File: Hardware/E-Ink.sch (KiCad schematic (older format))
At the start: 0 parts

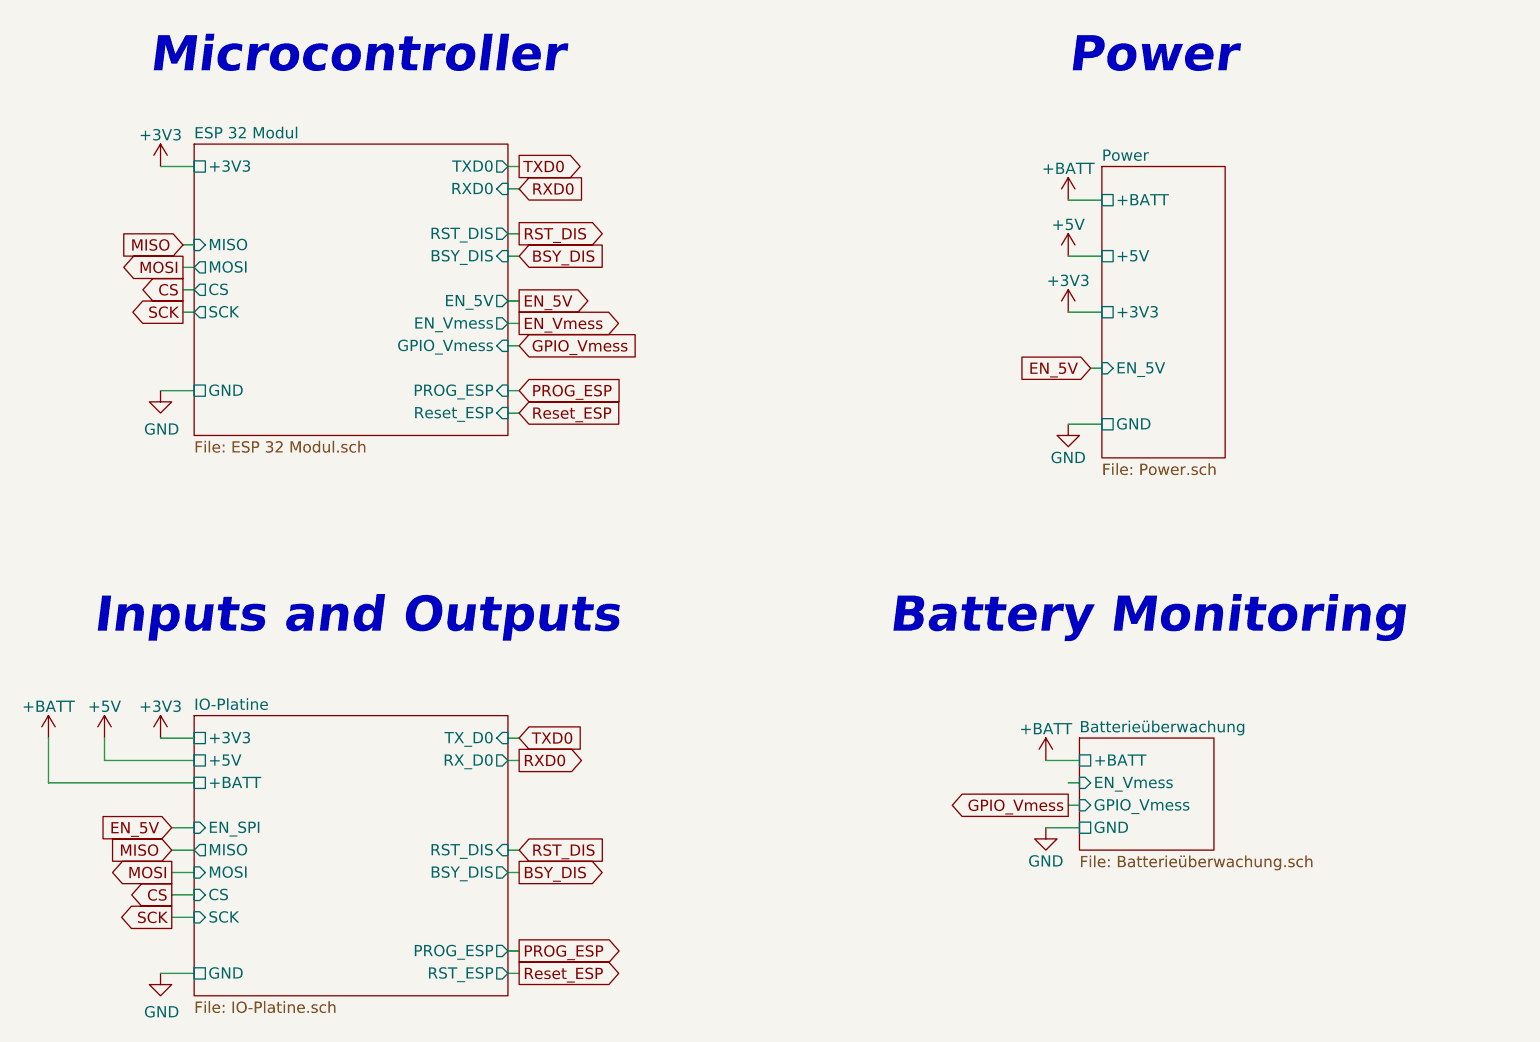
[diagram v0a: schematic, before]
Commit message: finished PCB, Thursday Review with Lukas
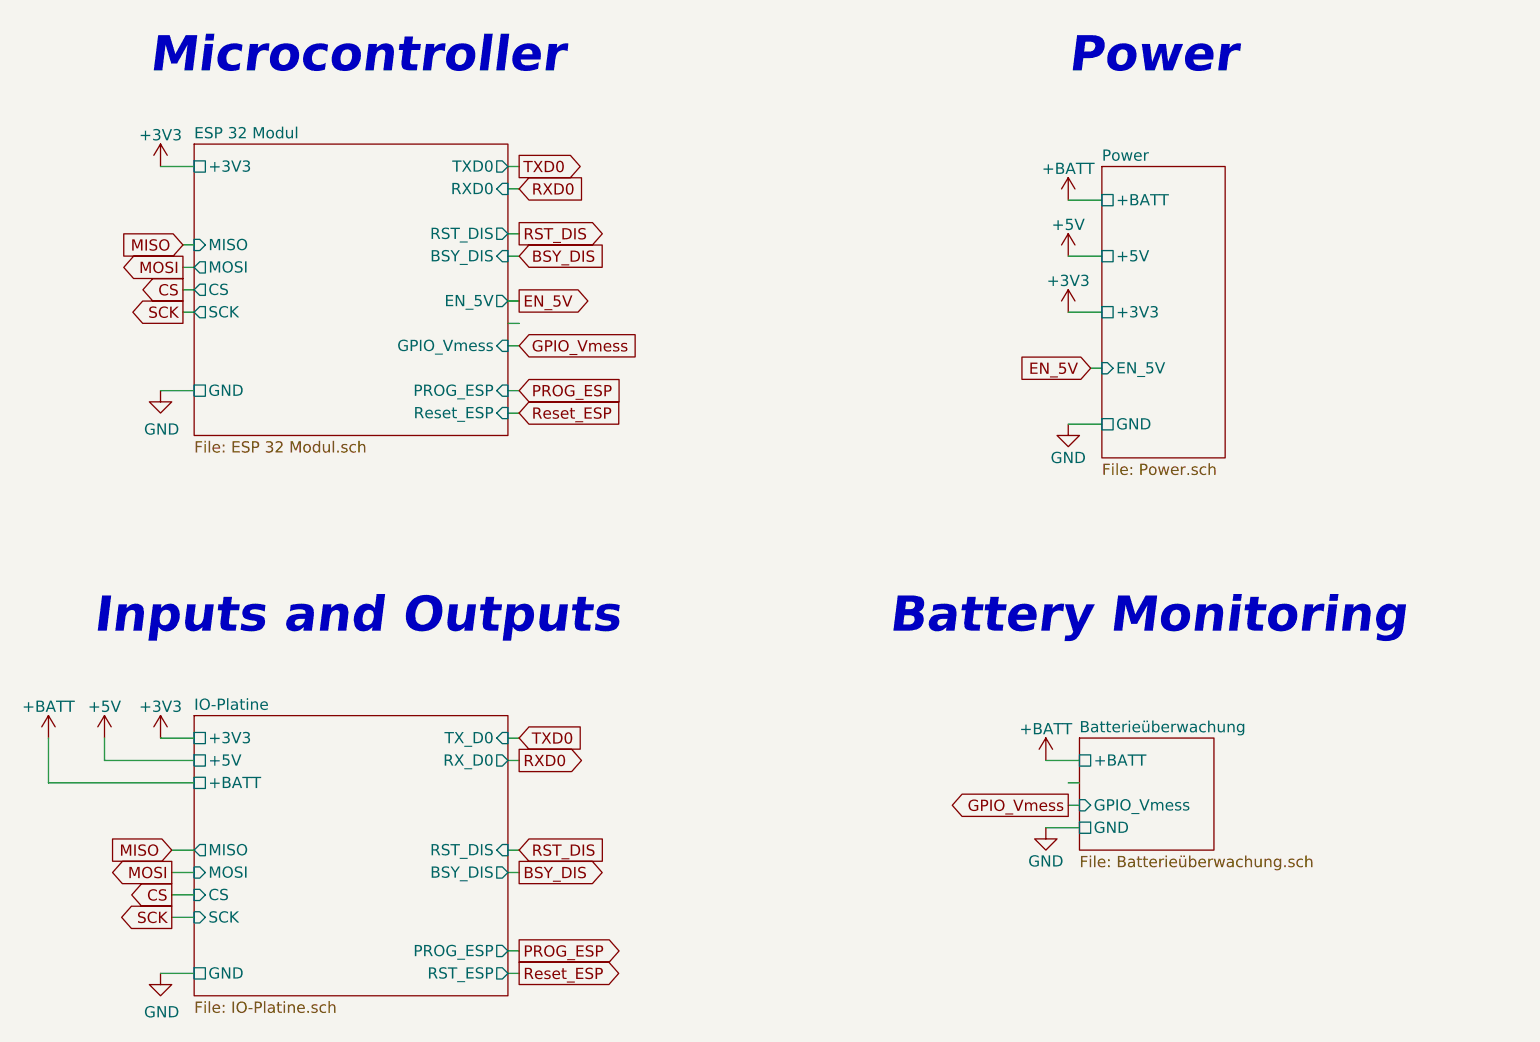
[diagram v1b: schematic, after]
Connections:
- net labels removed: EN_Vmess
- wire segments 41 -> 40
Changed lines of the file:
@@
 F0 "Batterieüberwachung" 50
 F1 "Batterieüberwachung.sch" 50
-F2 "EN_Vmess" I L 6900 5100 50
-F3 "+BATT" U L 6900 5000 50
-F4 "GPIO_Vmess" I L 6900 5200 50
-F5 "GND" U L 6900 5300 50
+F2 "+BATT" U L 6900 5000 50
+F3 "GPIO_Vmess" I L 6900 5200 50
+F4 "GND" U L 6900 5300 50
 $EndSheet
 $Comp
@@
 F8 "RXD0" I R 4350 2450 50
 F9 "EN_5V" O R 4350 2950 50
-F10 "EN_Vmess" O R 4350 3050 50
-F11 "CS" O L 2950 2900 50
-F12 "SCK" O L 2950 3000 50
-F13 "MOSI" O L 2950 2800 50
-F14 "PROG_ESP" I R 4350 3350 50
-F15 "RST_DIS" O R 4350 2650 50
-F16 "BSY_DIS" I R 4350 2750 50
+F10 "CS" O L 2950 2900 50
+F11 "SCK" O L 2950 3000 50
+F12 "MOSI" O L 2950 2800 50
+F13 "PROG_ESP" I R 4350 3350 50
+F14 "RST_DIS" O R 4350 2650 50
+F15 "BSY_DIS" I R 4350 2750 50
 $EndSheet
 $Comp
@@
 F0 "IO-Platine" 50
 F1 "IO-Platine.sch" 50
-F2 "EN_SPI" I L 2950 5300 50
-F3 "CS" I L 2950 5600 50
-F4 "SCK" I L 2950 5700 50
-F5 "MOSI" I L 2950 5500 50
-F6 "MISO" O L 2950 5400 50
-F7 "RST_ESP" O R 4350 5950 50
-F8 "+3V3" U L 2950 4900 50
-F9 "+5V" U L 2950 5000 50
-F10 "GND" U L 2950 5950 50
-F11 "RST_DIS" I R 4350 5400 50
-F12 "BSY_DIS" O R 4350 5500 50
-F13 "PROG_ESP" O R 4350 5850 50
-F14 "+BATT" U L 2950 5100 50
-F15 "RX_D0" O R 4350 5000 50
-F16 "TX_D0" I R 4350 4900 50
+F2 "CS" I L 2950 5600 50
+F3 "SCK" I L 2950 5700 50
+F4 "MOSI" I L 2950 5500 50
+F5 "MISO" O L 2950 5400 50
+F6 "RST_ESP" O R 4350 5950 50
+F7 "+3V3" U L 2950 4900 50
+F8 "+5V" U L 2950 5000 50
+F9 "GND" U L 2950 5950 50
+F10 "RST_DIS" I R 4350 5400 50
+F11 "BSY_DIS" O R 4350 5500 50
+F12 "PROG_ESP" O R 4350 5850 50
+F13 "+BATT" U L 2950 5100 50
+F14 "RX_D0" O R 4350 5000 50
+F15 "TX_D0" I R 4350 4900 50
 $EndSheet
 $Comp
@@
 Text GLabel 4400 2950 2    50   Output ~ 0
 EN_5V
-Text GLabel 4400 3050 2    50   Output ~ 0
-EN_Vmess
 Wire Wire Line
 	4400 2950 4350 2950
@@
 Wire Wire Line
 	4350 3450 4400 3450
-Text GLabel 2850 5300 0    50   Input ~ 0
-EN_5V
-Wire Wire Line
-	2850 5300 2950 5300
 $Comp
 L power:GND #PWR0104
